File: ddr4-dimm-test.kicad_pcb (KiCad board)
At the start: 2 copper layers, 133.3 x 31.2 mm, 137 parts, among them IC1 DDR4-BGA78, IC2 DDR4-BGA78, IC3 DDR4-BGA78, IC4 DDR4-BGA78, IC5 DDR4-BGA78, IC6 DDR4-BGA78, IC7 DDR4-BGA78, IC8 DDR4-BGA78

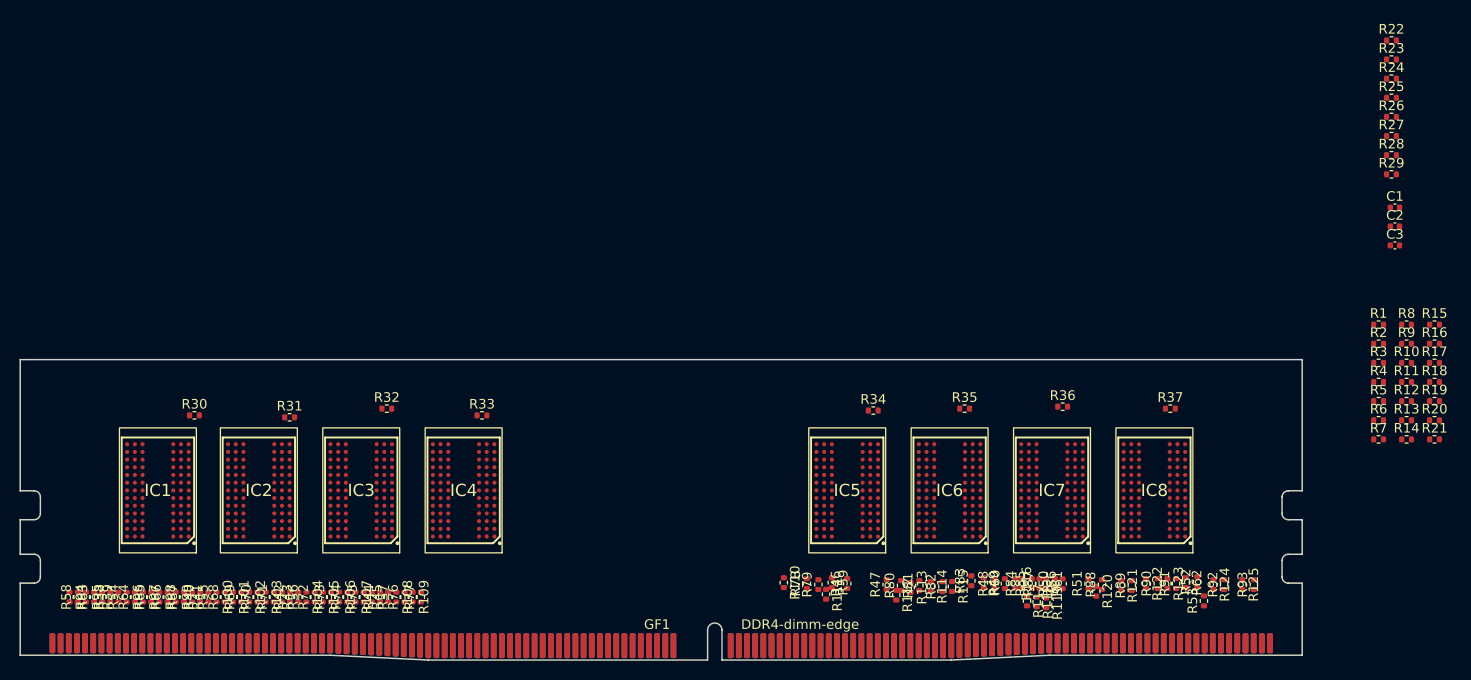
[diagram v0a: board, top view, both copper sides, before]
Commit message: Some more layout testing
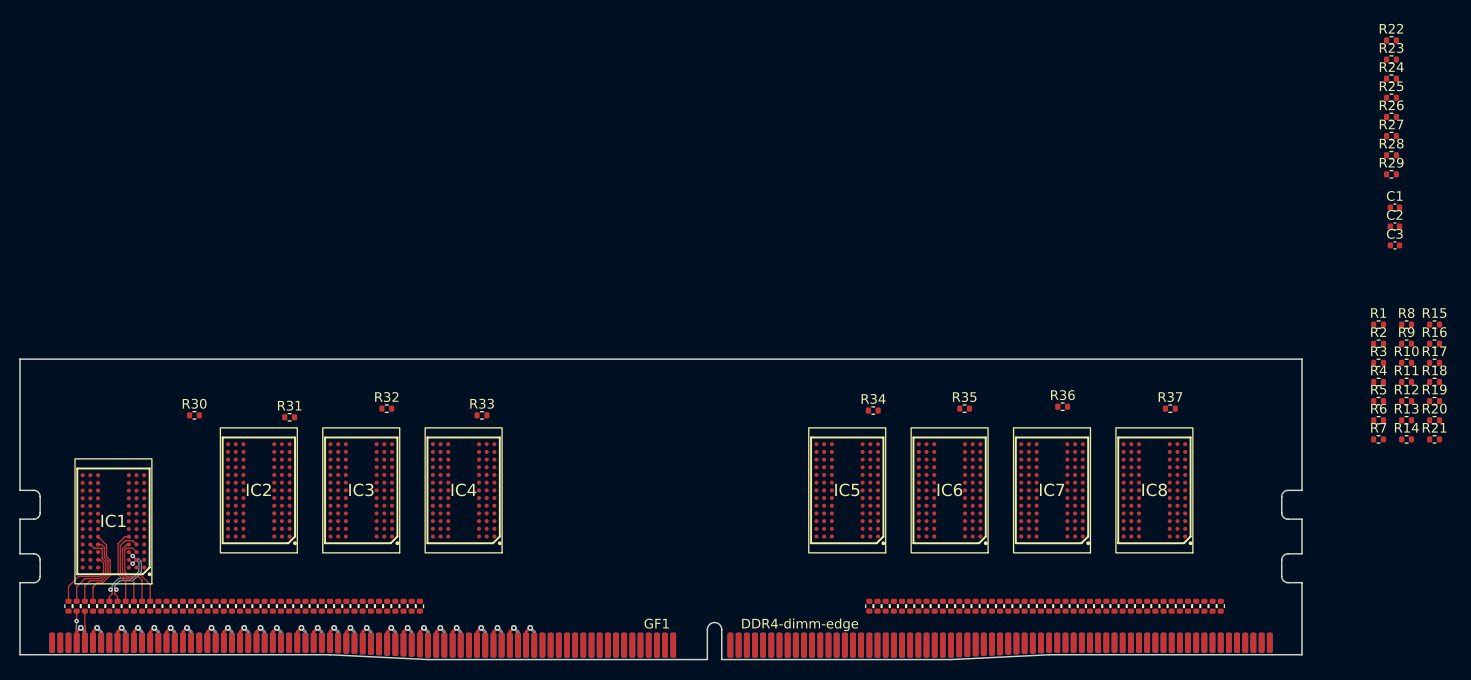
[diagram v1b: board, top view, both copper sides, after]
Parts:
- moved R110 9.23 mm to (163.7, 106.3)
- moved R79 8.17 mm to (166.2, 106.3)
- moved R78 7.72 mm to (164.6, 106.3)
- moved R59 7.70 mm to (167.1, 106.3)
- moved R46 6.96 mm to (167.9, 106.3)
- moved R111 6.32 mm to (165.4, 106.3)
- moved IC1 5.64 mm to (85.1, 97.5)
- moved R61 4.38 mm to (185.8, 106.3)
- moved R50 4.34 mm to (186.7, 106.3)
- moved R87 4.26 mm to (184.9, 106.3)
- moved R93 4.12 mm to (200.2, 106.3)
- moved R80 4.11 mm to (170.5, 106.3)
- moved R47 3.99 mm to (168.8, 106.3)
- moved R81 3.94 mm to (172.2, 106.3)
- moved R113 3.88 mm to (171.3, 106.3)
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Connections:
- IC1 pad B7: DQ1 -> DQ4
- IC1 pad C2: DQ0 -> DQ3
- IC1 pad D2: DQ4 -> DQ7
- IC1 pad D7: DQ3 -> DQ0
- IC1 pad E7: DQ7 -> DQ1
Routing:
- net GND: track 0.00 -> 91.6 mm, vias 0 -> 25
- net DQ5: track 0.00 -> 9.23 mm
- net DQ7: track 0.00 -> 8.69 mm
- net DQ3: track 0.00 -> 8.68 mm
- net DQ1: track 0.00 -> 8.32 mm
- net DQ0: track 0.00 -> 8.25 mm
- net DQS0+: track 0.00 -> 8.07 mm, vias 0 -> 2
- net DQ2: track 0.00 -> 7.86 mm
- net DQ6: track 0.00 -> 7.74 mm
- net DQS0-: track 0.00 -> 7.66 mm, vias 0 -> 2
- net DQ4: track 0.00 -> 7.50 mm
- net VDD: track 0.00 -> 3.95 mm, vias 0 -> 1
- net Net-(GF1-DQ5): track 0.00 -> 3.33 mm, vias 0 -> 1
- net Net-(GF1-DQ0): track 0.00 -> 3.33 mm
